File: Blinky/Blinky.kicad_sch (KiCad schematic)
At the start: 17 parts, among them IC1 PAM8303CBSC, J1 TP4056, J2 Battery Connector, J3 Speaker Connector, J4 USB_B_Micro, J5 Charging Notches, SW1 SW_Push, U1 ESP32-S2-WROVER

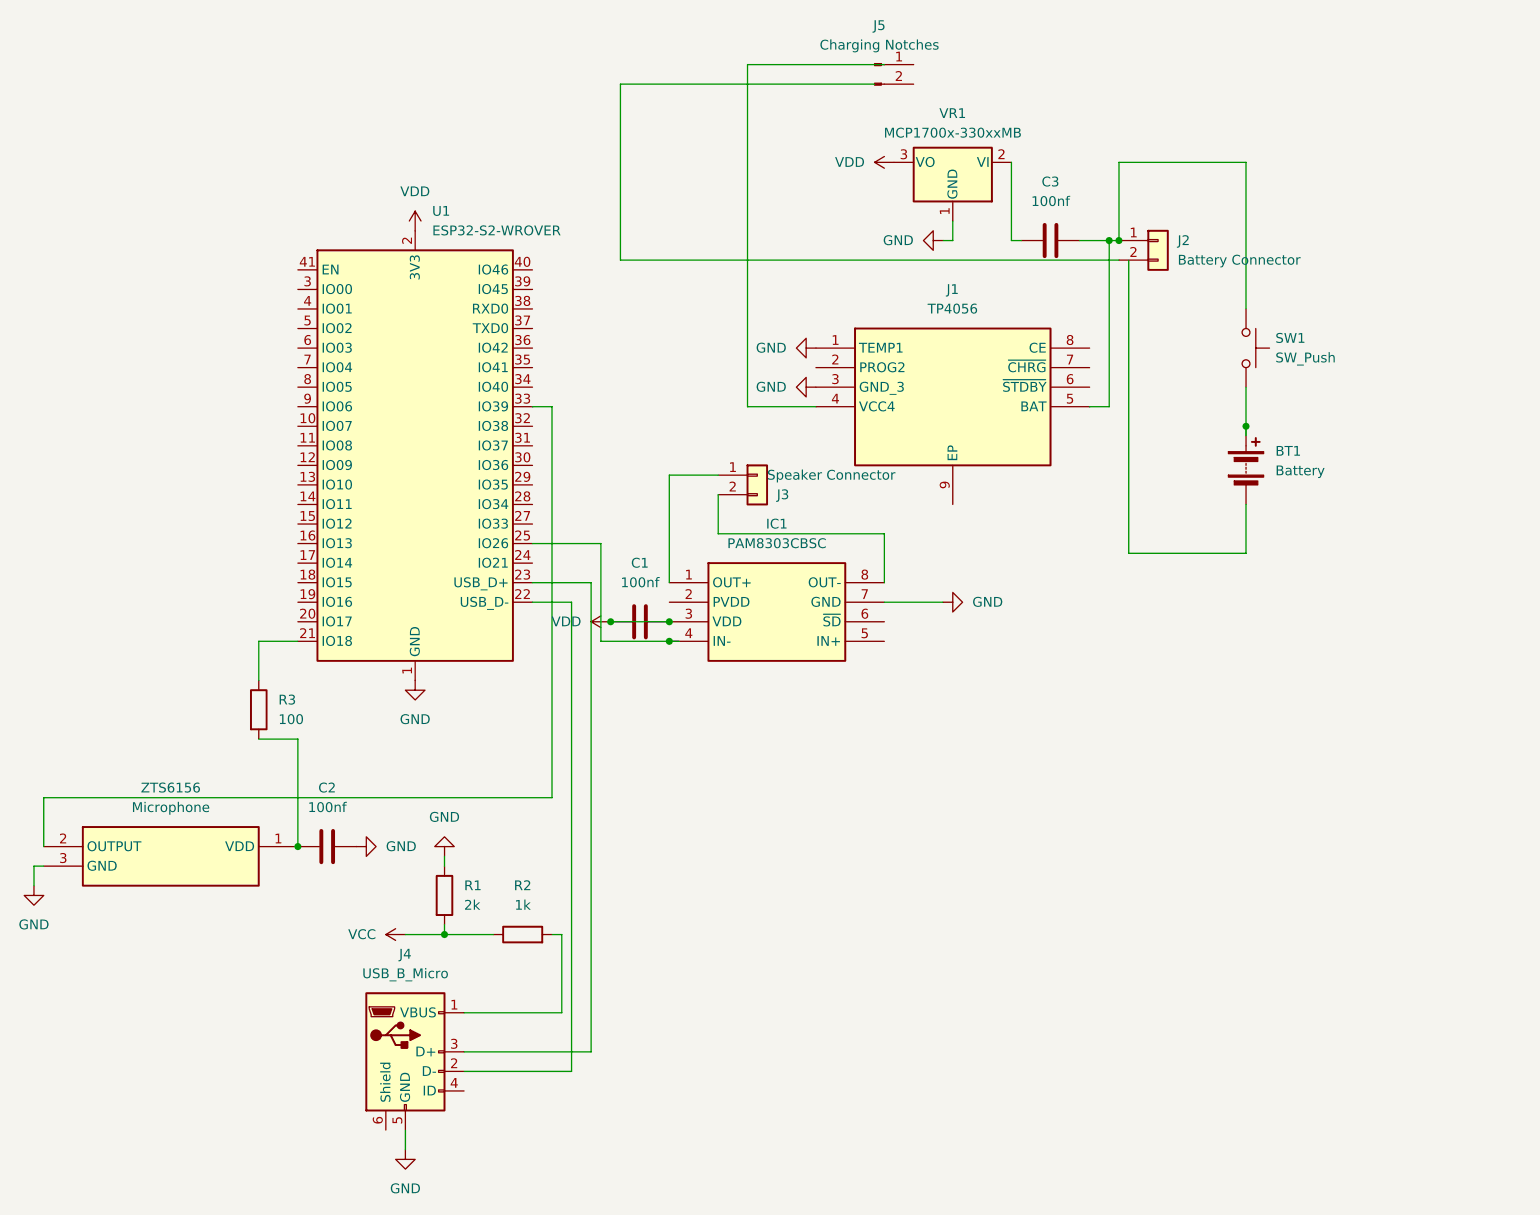
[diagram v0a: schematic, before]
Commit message: bugfix
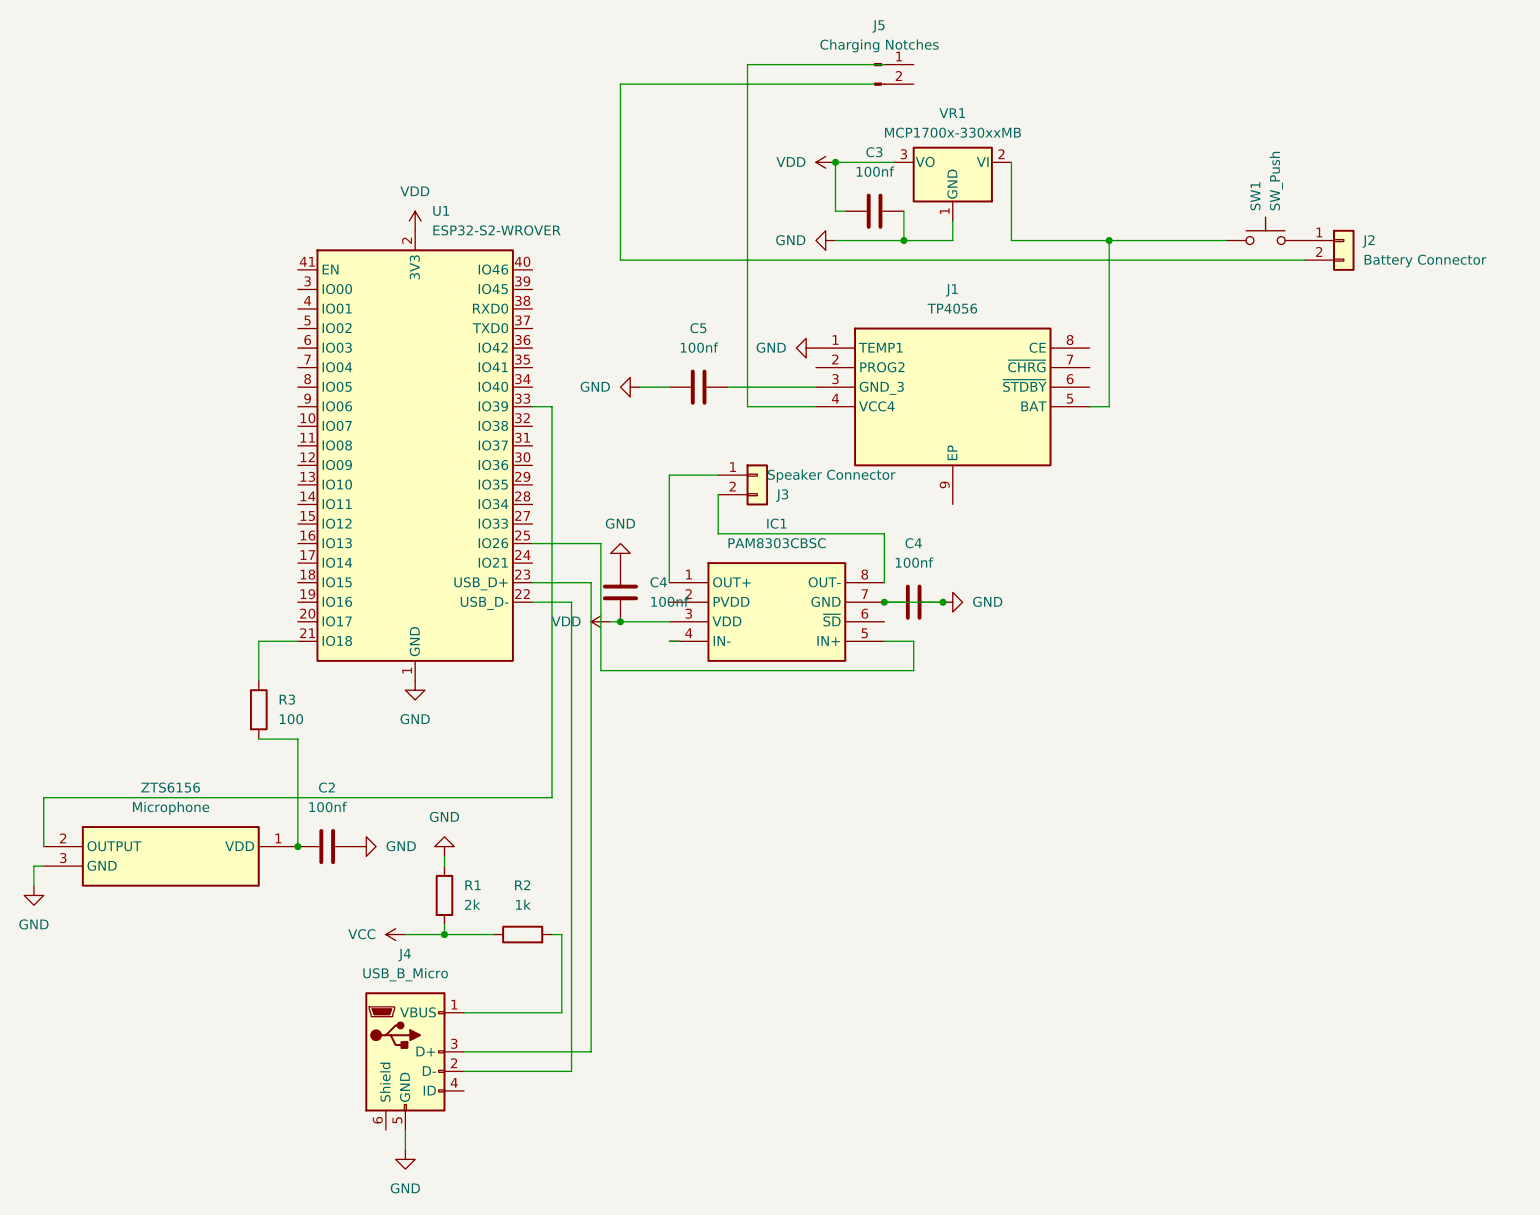
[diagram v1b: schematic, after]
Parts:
- removed BT1: Battery, symbol Device:Battery
- removed C1: 100nf, symbol Device:C
- added C4 (x2), C5: 100nf, symbol Device:C
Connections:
- net GND: now also C3.2, C4.1, C4.2, C4.2, C5.1; no longer J1.3 (GND_3)
- net VDD: now also C3.1, C4.1
- net at J1.5 (BAT), SW1.1: now also VR1.2 (VI); no longer C3.2, J2.1 (Pin_1)
- net at SW1.2: now also J2.1 (Pin_1)
- net at U1.25 (IO26): now also IC1.5 (IN+); no longer IC1.4 (IN-)
- new net: C5.2, J1.3 (GND_3)
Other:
- moved on the sheet: J2, SW1
